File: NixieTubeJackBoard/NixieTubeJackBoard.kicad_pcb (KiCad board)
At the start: 2 copper layers, 17.1 x 17.1 mm, 2 parts, among them J1 Conn_01x13_Male, J2 Conn_01x13_Female

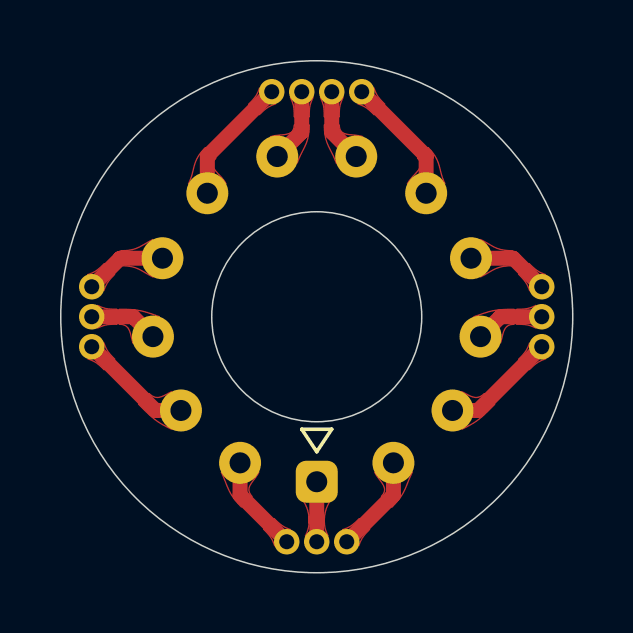
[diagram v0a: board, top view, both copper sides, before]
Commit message: 拆分得七零八落
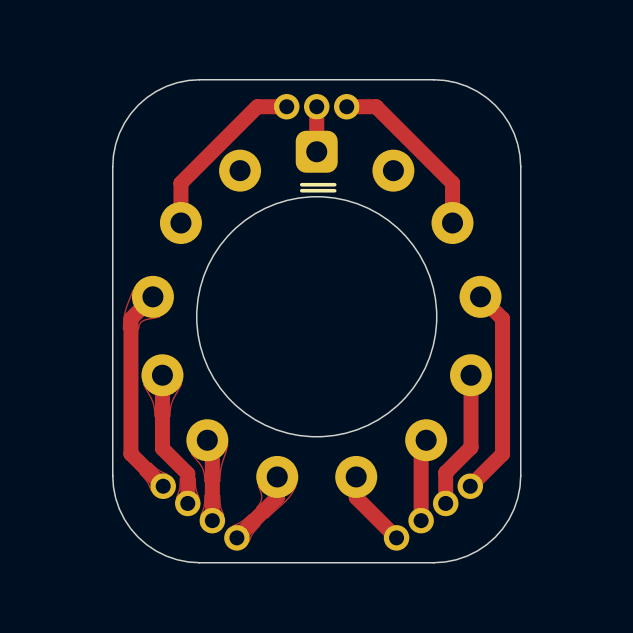
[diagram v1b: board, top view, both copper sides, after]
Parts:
- turned J1 to 180 degrees
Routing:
- net Net-(J1-Pad4): track 2.31 -> 7.06 mm
- net Net-(J1-Pad11): track 2.31 -> 7.06 mm
- net Net-(J1-Pad2): track 3.27 -> 0.00 mm
- net Net-(J1-Pad13): track 3.27 -> 0.00 mm
- net Net-(J1-Pad3): track 3.85 -> 5.91 mm
- net Net-(J1-Pad12): track 3.85 -> 5.91 mm
- net Net-(J1-Pad5): track 2.75 -> 4.62 mm
- net Net-(J1-Pad10): track 2.75 -> 4.62 mm
- net Net-(J1-Pad9): track 4.27 -> 2.75 mm
- net Net-(J1-Pad6): track 4.27 -> 2.75 mm
- net Net-(J1-Pad1): track 2.00 -> 1.50 mm
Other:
- board size 17.1 x 17.1 mm -> 13.6 x 16.1 mm
